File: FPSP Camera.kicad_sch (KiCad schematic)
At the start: 78 parts, among them J1 Conn_01x24_Socket, J2 Conn_02x04_Counter_Clockwise, J3 Conn_02x07_Counter_Clockwise, J4 SM03B-SRSS-TB, J5 USB_B_Micro, J6 Conn_02x06_Odd_Even, U1 ICM-45686, U2 W25Q128JVS, U3 RP2350_60QFN, U4 TLV75533PDRV, U5 TLV73328PDRV, U6 TLV73315PDRV, Y1 SiT8008xx-1x-xxE

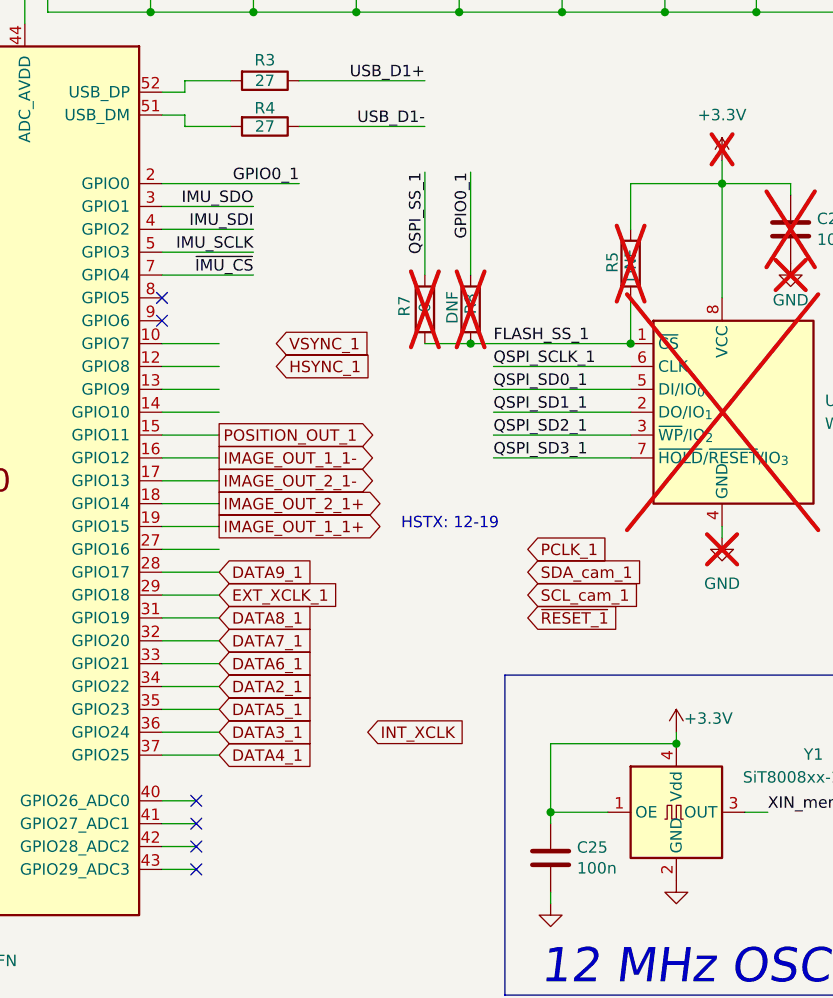
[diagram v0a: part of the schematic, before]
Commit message: pin assignment done
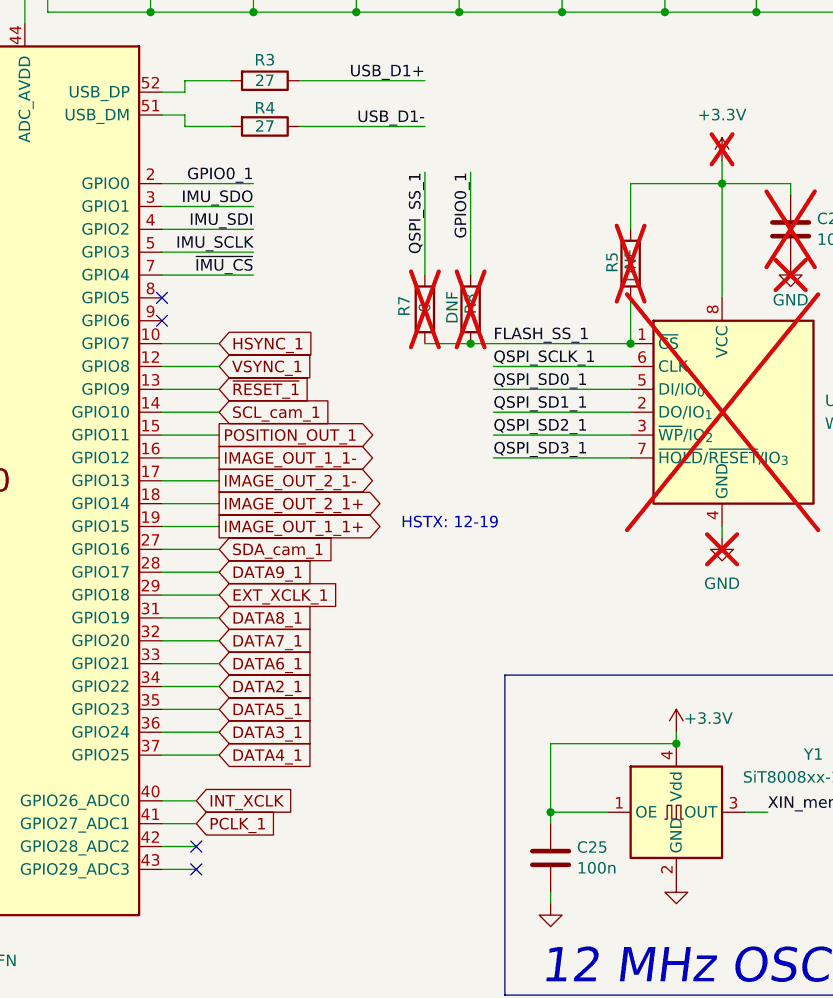
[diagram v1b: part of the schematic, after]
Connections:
- net HSYNC_1: now also U3.10 (GPIO7)
- net INT_XCLK: now also U3.40 (GPIO26_ADC0)
- net PCLK_1: now also U3.41 (GPIO27_ADC1)
- net SCL_cam_1: now also U3.14 (GPIO10)
- net SDA_cam_1: now also U3.27 (GPIO16)
- net VSYNC_1: now also U3.12 (GPIO8)
- net ~{RESET_1}: now also U3.13 (GPIO9)
- no-connect marks 36 -> 34
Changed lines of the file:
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@@
 	)
 	(no_connect
-		(at 157.48 154.94)
-	)
-	(no_connect
 		(at 74.295 312.42)
 	)
@@
 	)
 	(no_connect
-		(at 157.48 157.48)
-	)
-	(no_connect
 		(at 112.395 316.23)
 	)
@@
 	(wire
 		(pts
-			(xy 153.67 86.36) (xy 168.91 86.36)
+			(xy 153.67 86.36) (xy 163.83 86.36)
 		)
 		(stroke
@@
 	)
 	(label "GPIO0_1"
-		(at 168.91 86.36 180)
+		(at 163.83 86.36 180)
 		(effects
 			(font
@@
 		)
 	)
-	(global_label "DATA5_1"
-		(shape output)
-		(at 271.78 149.86 0)
+	(global_label "~{RESET_1}"
+		(shape input)
+		(at 160.02 109.22 0)
 		(fields_autoplaced yes)
 		(effects
@@
 		)
 		(property "Intersheetrefs" "${INTERSHEET_REFS}"
-			(at 282.5666 149.86 0)
+			(at 170.9274 109.22 0)
 			(effects
 				(font
@@
 		)
 	)
-	(global_label "DATA2_1"
+	(global_label "DATA5_1"
 		(shape output)
-		(at 271.78 147.32 0)
+		(at 271.78 149.86 0)
 		(fields_autoplaced yes)
 		(effects
@@
 		)
 		(property "Intersheetrefs" "${INTERSHEET_REFS}"
-			(at 282.5666 147.32 0)
+			(at 282.5666 149.86 0)
 			(effects
 				(font
@@
 		)
 	)
-	(global_label "~{RESET_1}"
-		(shape input)
-		(at 194.31 134.62 0)
+	(global_label "DATA2_1"
+		(shape output)
+		(at 271.78 147.32 0)
 		(fields_autoplaced yes)
 		(effects
@@
 		)
 		(property "Intersheetrefs" "${INTERSHEET_REFS}"
-			(at 205.2174 134.62 0)
+			(at 282.5666 147.32 0)
 			(effects
 				(font
@@
 		)
 	)
-	(global_label "SWD_1"
+	(global_label "SCL_cam_1"
 		(shape input)
-		(at 158.75 321.31 180)
+		(at 160.02 111.76 0)
 		(fields_autoplaced yes)
 		(effects
@@
 				(size 1.27 1.27)
 			)
-			(justify right)
+			(justify left)
 		)
 		(property "Intersheetrefs" "${INTERSHEET_REFS}"
-			(at 149.6568 321.31 0)
+			(at 173.5884 111.76 0)
 			(effects
 				(font
 					(size 1.27 1.27)
 				)
-				(justify right)
+				(justify left)
 				(hide yes)
 			)
 		)
 	)
-	(global_label "SDA_cam_1"
+	(global_label "SWD_1"
 		(shape input)
-		(at 194.31 129.54 0)
+		(at 158.75 321.31 180)
 		(fields_autoplaced yes)
 		(effects
@@
 				(size 1.27 1.27)
 			)
-			(justify left)
+			(justify right)
 		)
 		(property "Intersheetrefs" "${INTERSHEET_REFS}"
-			(at 207.9389 129.54 0)
+			(at 149.6568 321.31 0)
 			(effects
 				(font
 					(size 1.27 1.27)
 				)
-				(justify left)
+				(justify right)
 				(hide yes)
 			)
@@
 	(global_label "INT_XCLK"
 		(shape input)
-		(at 176.53 147.32 0)
+		(at 157.48 154.94 0)
 		(fields_autoplaced yes)
 		(effects
@@
 		)
 		(property "Intersheetrefs" "${INTERSHEET_REFS}"
-			(at 188.1633 147.32 0)
+			(at 169.1133 154.94 0)
 			(effects
 				(font
@@
 		)
 	)
-	(global_label "VSYNC_1"
-		(shape input)
-		(at 166.37 104.14 0)
-		(fields_autoplaced yes)
-		(effects
-			(font
-				(size 1.27 1.27)
-			)
-			(justify left)
-		)
-		(property "Intersheetrefs" "${INTERSHEET_REFS}"
-			(at 177.5195 104.14 0)
-			(effects
-				(font
-					(size 1.27 1.27)
-				)
-				(justify left)
-				(hide yes)
-			)
-		)
-	)
 	(global_label "DATA7_1"
 		(shape output)
@@
 	(global_label "PCLK_1"
 		(shape input)
-		(at 194.31 127 0)
+		(at 157.48 157.48 0)
 		(fields_autoplaced yes)
 		(effects
@@
 		)
 		(property "Intersheetrefs" "${INTERSHEET_REFS}"
-			(at 204.3104 127 0)
+			(at 167.4804 157.48 0)
 			(effects
 				(font
@@
 		)
 	)
-	(global_label "SCL_cam_1"
-		(shape input)
-		(at 194.31 132.08 0)
+	(global_label "DGND"
+		(shape bidirectional)
+		(at 350.52 102.87 90)
 		(fields_autoplaced yes)
 		(effects
@@
 		)
 		(property "Intersheetrefs" "${INTERSHEET_REFS}"
-			(at 207.8784 132.08 0)
+			(at 350.52 93.633 90)
 			(effects
 				(font
@@
 		)
 	)
-	(global_label "DGND"
-		(shape bidirectional)
-		(at 350.52 102.87 90)
+	(global_label "IMAGE_OUT_1_1"
+		(shape input)
+		(at 128.905 316.23 0)
 		(fields_autoplaced yes)
 		(effects
@@
 		)
 		(property "Intersheetrefs" "${INTERSHEET_REFS}"
-			(at 350.52 93.633 90)
+			(at 146.4044 316.23 0)
 			(effects
 				(font
@@
 		)
 	)
-	(global_label "IMAGE_OUT_1_1"
-		(shape input)
-		(at 128.905 316.23 0)
+	(global_label "DATA0_1"
+		(shape output)
+		(at 271.78 160.02 0)
 		(fields_autoplaced yes)
 		(effects
@@
 		)
 		(property "Intersheetrefs" "${INTERSHEET_REFS}"
-			(at 146.4044 316.23 0)
+			(at 282.5666 160.02 0)
 			(effects
 				(font
@@
 		)
 	)
-	(global_label "DATA0_1"
-		(shape output)
-		(at 271.78 160.02 0)
+	(global_label "HSYNC_1"
+		(shape input)
+		(at 160.02 104.14 0)
 		(fields_autoplaced yes)
 		(effects
@@
 		)
 		(property "Intersheetrefs" "${INTERSHEET_REFS}"
-			(at 282.5666 160.02 0)
+			(at 171.4114 104.14 0)
 			(effects
 				(font
@@
 		)
 	)
-	(global_label "HSYNC_1"
+	(global_label "SDA_cam_1"
+		(shape input)
+		(at 160.02 127 0)
+		(fields_autoplaced yes)
+		(effects
+			(font
+				(size 1.27 1.27)
+			)
+			(justify left)
+		)
+		(property "Intersheetrefs" "${INTERSHEET_REFS}"
+			(at 173.6489 127 0)
+			(effects
+				(font
+					(size 1.27 1.27)
+				)
+				(justify left)
+				(hide yes)
+			)
+		)
+	)
+	(global_label "VSYNC_1"
 		(shape input)
-		(at 166.37 106.68 0)
+		(at 160.02 106.68 0)
 		(fields_autoplaced yes)
 		(effects
@@
 		)
 		(property "Intersheetrefs" "${INTERSHEET_REFS}"
-			(at 177.7614 106.68 0)
+			(at 171.1695 106.68 0)
 			(effects
 				(font

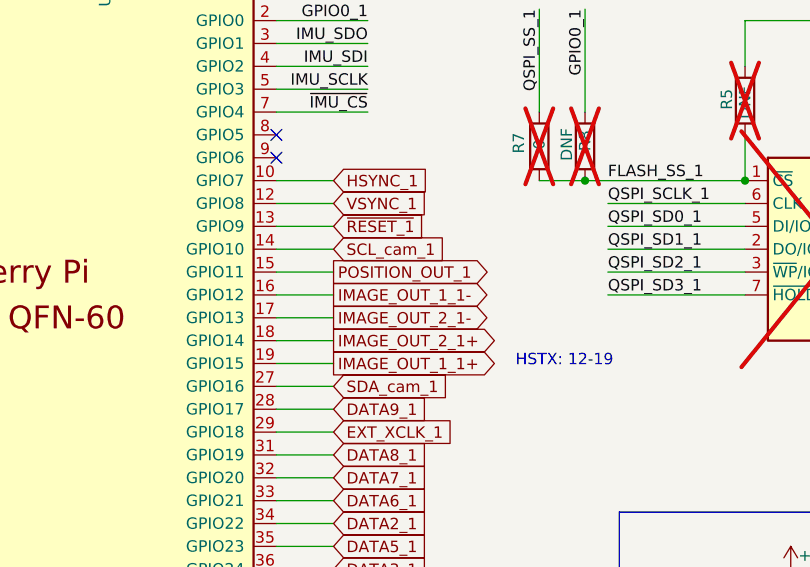
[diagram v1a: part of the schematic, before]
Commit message: finished connecting all data pins
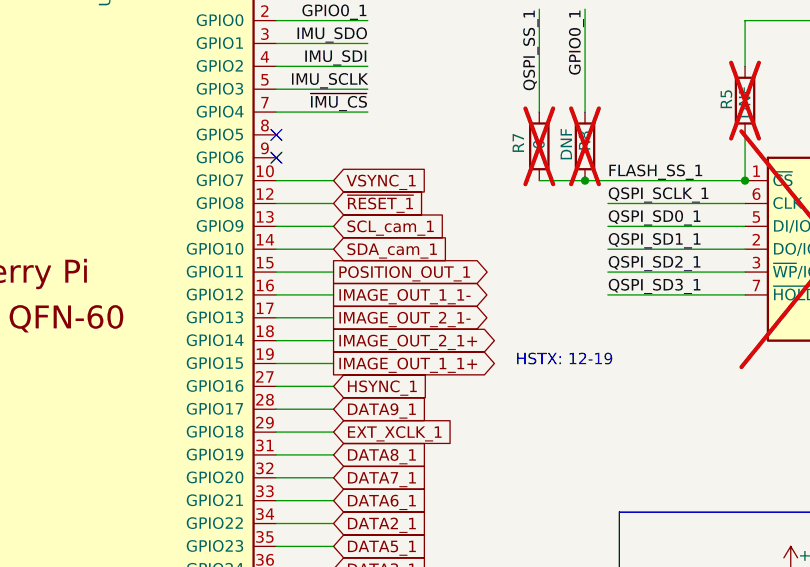
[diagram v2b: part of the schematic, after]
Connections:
- net HSYNC_1: now also U3.27 (GPIO16); no longer U3.10 (GPIO7)
- net SCL_cam_1: now also U3.13 (GPIO9); no longer U3.14 (GPIO10)
- net SDA_cam_1: now also U3.14 (GPIO10); no longer U3.27 (GPIO16)
- net VSYNC_1: now also U3.10 (GPIO7); no longer U3.12 (GPIO8)
- net ~{RESET_1}: now also U3.12 (GPIO8); no longer U3.13 (GPIO9)
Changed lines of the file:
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@@
 	(global_label "~{RESET_1}"
 		(shape input)
-		(at 160.02 109.22 0)
-		(fields_autoplaced yes)
-		(effects
-			(font
-				(size 1.27 1.27)
-			)
-			(justify left)
-		)
-		(property "Intersheetrefs" "${INTERSHEET_REFS}"
-			(at 170.9274 109.22 0)
+		(at 160.02 106.68 0)
+		(fields_autoplaced yes)
+		(effects
+			(font
+				(size 1.27 1.27)
+			)
+			(justify left)
+		)
+		(property "Intersheetrefs" "${INTERSHEET_REFS}"
+			(at 170.9274 106.68 0)
 			(effects
 				(font
@@
 	(global_label "SCL_cam_1"
 		(shape input)
-		(at 160.02 111.76 0)
-		(fields_autoplaced yes)
-		(effects
-			(font
-				(size 1.27 1.27)
-			)
-			(justify left)
-		)
-		(property "Intersheetrefs" "${INTERSHEET_REFS}"
-			(at 173.5884 111.76 0)
+		(at 160.02 109.22 0)
+		(fields_autoplaced yes)
+		(effects
+			(font
+				(size 1.27 1.27)
+			)
+			(justify left)
+		)
+		(property "Intersheetrefs" "${INTERSHEET_REFS}"
+			(at 173.5884 109.22 0)
 			(effects
 				(font
@@
 	(global_label "HSYNC_1"
 		(shape input)
+		(at 160.02 127 0)
+		(fields_autoplaced yes)
+		(effects
+			(font
+				(size 1.27 1.27)
+			)
+			(justify left)
+		)
+		(property "Intersheetrefs" "${INTERSHEET_REFS}"
+			(at 171.4114 127 0)
+			(effects
+				(font
+					(size 1.27 1.27)
+				)
+				(justify left)
+				(hide yes)
+			)
+		)
+	)
+	(global_label "DATA1_1"
+		(shape output)
+		(at 271.78 157.48 0)
+		(fields_autoplaced yes)
+		(effects
+			(font
+				(size 1.27 1.27)
+			)
+			(justify left)
+		)
+		(property "Intersheetrefs" "${INTERSHEET_REFS}"
+			(at 282.5666 157.48 0)
+			(effects
+				(font
+					(size 1.27 1.27)
+				)
+				(justify left)
+				(hide yes)
+			)
+		)
+	)
+	(global_label "IMAGE_OUT_1_1+"
+		(shape output)
+		(at 160.02 124.46 0)
+		(fields_autoplaced yes)
+		(effects
+			(font
+				(size 1.27 1.27)
+			)
+			(justify left)
+		)
+		(property "Intersheetrefs" "${INTERSHEET_REFS}"
+			(at 179.0918 124.46 0)
+			(effects
+				(font
+					(size 1.27 1.27)
+				)
+				(justify left)
+				(hide yes)
+			)
+		)
+	)
+	(global_label "EXT_XCLK_1"
+		(shape input)
+		(at 298.45 129.54 0)
+		(fields_autoplaced yes)
+		(effects
+			(font
+				(size 1.27 1.27)
+			)
+			(justify left)
+		)
+		(property "Intersheetrefs" "${INTERSHEET_REFS}"
+			(at 312.6836 129.54 0)
+			(effects
+				(font
+					(size 1.27 1.27)
+				)
+				(justify left)
+				(hide yes)
+			)
+		)
+	)
+	(global_label "DATA3_1"
+		(shape output)
+		(at 271.78 152.4 0)
+		(fields_autoplaced yes)
+		(effects
+			(font
+				(size 1.27 1.27)
+			)
+			(justify left)
+		)
+		(property "Intersheetrefs" "${INTERSHEET_REFS}"
+			(at 282.5666 152.4 0)
+			(effects
+				(font
+					(size 1.27 1.27)
+				)
+				(justify left)
+				(hide yes)
+			)
+		)
+	)
+	(global_label "SDA_cam_1"
+		(shape input)
+		(at 160.02 111.76 0)
+		(fields_autoplaced yes)
+		(effects
+			(font
+				(size 1.27 1.27)
+			)
+			(justify left)
+		)
+		(property "Intersheetrefs" "${INTERSHEET_REFS}"
+			(at 173.6489 111.76 0)
+			(effects
+				(font
+					(size 1.27 1.27)
+				)
+				(justify left)
+				(hide yes)
+			)
+		)
+	)
+	(global_label "VSYNC_1"
+		(shape input)
 		(at 160.02 104.14 0)
 		(fields_autoplaced yes)
@@
 		)
 		(property "Intersheetrefs" "${INTERSHEET_REFS}"
-			(at 171.4114 104.14 0)
-			(effects
-				(font
-					(size 1.27 1.27)
-				)
-				(justify left)
-				(hide yes)
-			)
-		)
-	)
-	(global_label "DATA1_1"
-		(shape output)
-		(at 271.78 157.48 0)
-		(fields_autoplaced yes)
-		(effects
-			(font
-				(size 1.27 1.27)
-			)
-			(justify left)
-		)
-		(property "Intersheetrefs" "${INTERSHEET_REFS}"
-			(at 282.5666 157.48 0)
-			(effects
-				(font
-					(size 1.27 1.27)
-				)
-				(justify left)
-				(hide yes)
-			)
-		)
-	)
-	(global_label "IMAGE_OUT_1_1+"
-		(shape output)
-		(at 160.02 124.46 0)
-		(fields_autoplaced yes)
-		(effects
-			(font
-				(size 1.27 1.27)
-			)
-			(justify left)
-		)
-		(property "Intersheetrefs" "${INTERSHEET_REFS}"
-			(at 179.0918 124.46 0)
-			(effects
-				(font
-					(size 1.27 1.27)
-				)
-				(justify left)
-				(hide yes)
-			)
-		)
-	)
-	(global_label "EXT_XCLK_1"
-		(shape input)
-		(at 298.45 129.54 0)
-		(fields_autoplaced yes)
-		(effects
-			(font
-				(size 1.27 1.27)
-			)
-			(justify left)
-		)
-		(property "Intersheetrefs" "${INTERSHEET_REFS}"
-			(at 312.6836 129.54 0)
-			(effects
-				(font
-					(size 1.27 1.27)
-				)
-				(justify left)
-				(hide yes)
-			)
-		)
-	)
-	(global_label "DATA3_1"
-		(shape output)
-		(at 271.78 152.4 0)
-		(fields_autoplaced yes)
-		(effects
-			(font
-				(size 1.27 1.27)
-			)
-			(justify left)
-		)
-		(property "Intersheetrefs" "${INTERSHEET_REFS}"
-			(at 282.5666 152.4 0)
-			(effects
-				(font
-					(size 1.27 1.27)
-				)
-				(justify left)
-				(hide yes)
-			)
-		)
-	)
-	(global_label "SDA_cam_1"
-		(shape input)
-		(at 160.02 127 0)
-		(fields_autoplaced yes)
-		(effects
-			(font
-				(size 1.27 1.27)
-			)
-			(justify left)
-		)
-		(property "Intersheetrefs" "${INTERSHEET_REFS}"
-			(at 173.6489 127 0)
-			(effects
-				(font
-					(size 1.27 1.27)
-				)
-				(justify left)
-				(hide yes)
-			)
-		)
-	)
-	(global_label "VSYNC_1"
-		(shape input)
-		(at 160.02 106.68 0)
-		(fields_autoplaced yes)
-		(effects
-			(font
-				(size 1.27 1.27)
-			)
-			(justify left)
-		)
-		(property "Intersheetrefs" "${INTERSHEET_REFS}"
-			(at 171.1695 106.68 0)
-			(effects
-				(font
+			(at 171.1695 104.14 0)
+			(effects
+				(font
